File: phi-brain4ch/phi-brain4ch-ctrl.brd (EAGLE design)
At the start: 114.3 x 38.1 mm, 24 parts, among them U1 LCD-HD447804-HOLES16X2-4-HOLES

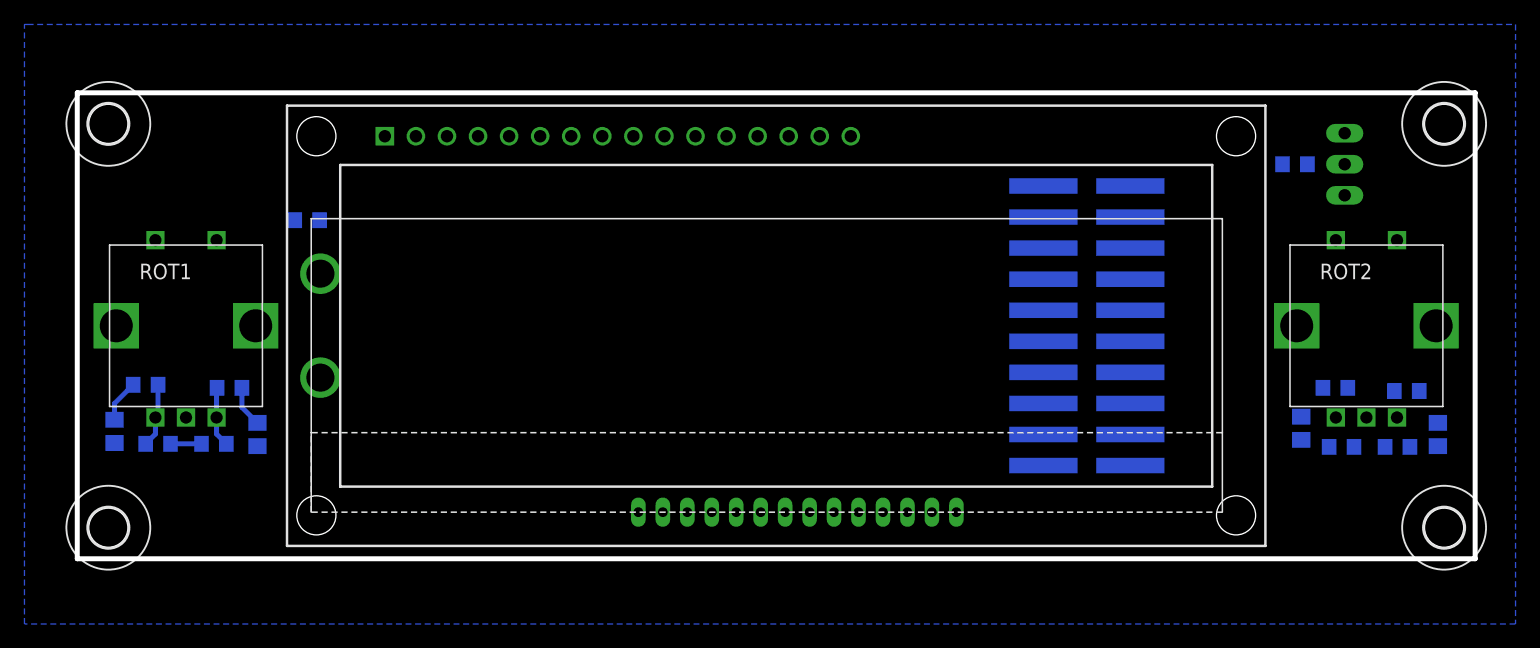
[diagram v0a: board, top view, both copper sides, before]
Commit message: wip
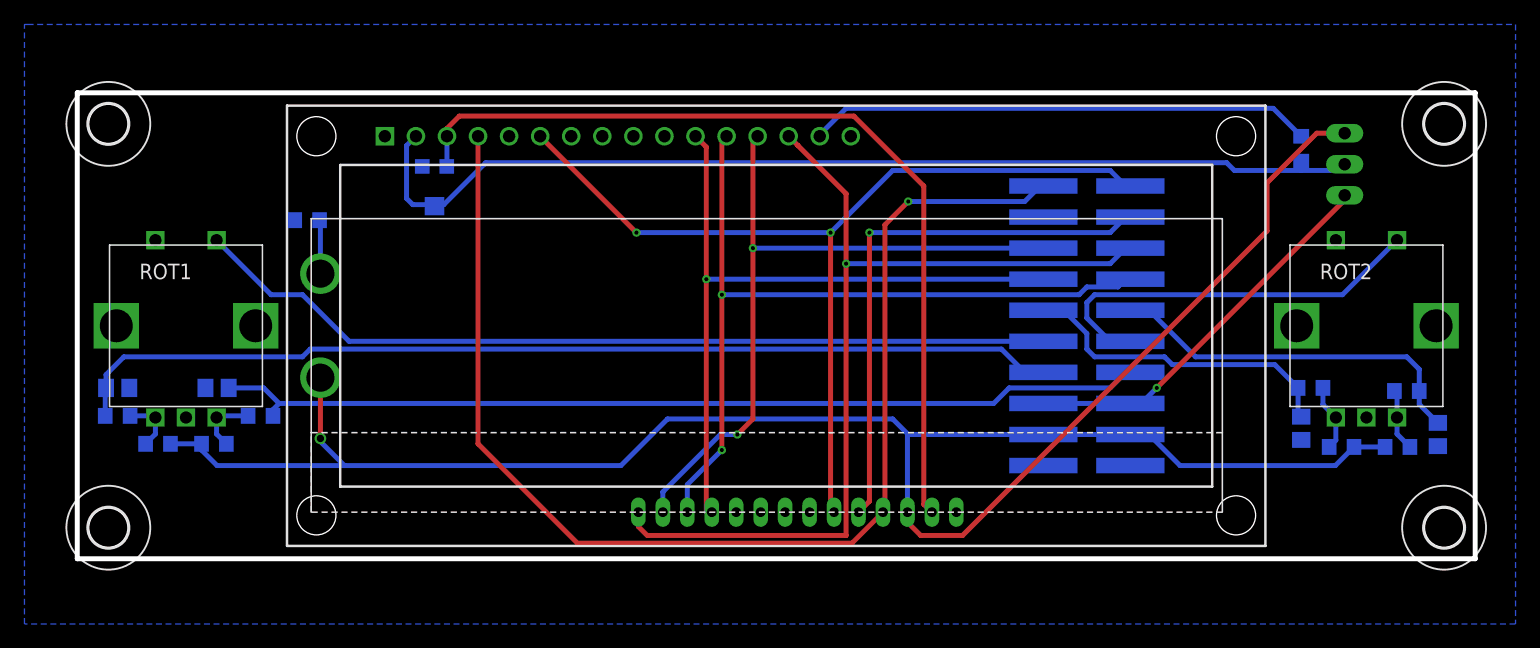
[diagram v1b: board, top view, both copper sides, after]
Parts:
- added VR1: 3303W-3-103E, microbuilder:TRIMPOT_BOURNS3MM
- moved C1 5.04 mm to (11.4, 14.0), turned to 0 degrees
- moved C2 3.57 mm to (3.30, 14.0), turned to 180 degrees
- moved R1 3.42 mm to (15.0, 11.7)
- moved R5 3.42 mm to (3.30, 11.7)
- moved R9 2.03 mm to (100.8, 14.0)
- moved R10 1.37 mm to (100.1, 33.5), turned to 270 degrees
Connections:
- net GND: now also VR1.A
- net LCD_V0: now also VR1.S
- net LCD_VDD: now also VR1.E
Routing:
- net 3.3V: track 2.54 -> 171.5 mm, vias 0 -> 1
- net LCD_RS: track 0.00 -> 100.5 mm, vias 0 -> 1
- net LCD_VDD: track 0.00 -> 85.2 mm
- net ROT1_A: track 3.49 -> 81.7 mm
- net LCD_EN: track 0.00 -> 77.1 mm, vias 0 -> 2
- net LCD_D7: track 0.00 -> 76.8 mm, vias 0 -> 1
- net ROT1_B: track 3.39 -> 76.5 mm
- net LCD_V0: track 0.00 -> 71.8 mm
- net ROT1_SW: track 0.00 -> 71.0 mm
- net LCD_D5: track 0.00 -> 66.0 mm, vias 0 -> 2
- net LCD_D4: track 0.00 -> 59.1 mm, vias 0 -> 1
- net LCD_D6: track 0.00 -> 58.5 mm, vias 0 -> 2
- net LCD_RW: track 0.00 -> 45.1 mm, vias 0 -> 1
- net N$6: track 0.00 -> 41.3 mm
- net ROT2_SW: track 0.00 -> 33.1 mm
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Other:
- board text added: "Designed by Eran Rundstein"
- board text added: "phi-brain-4ch-ctrl revision 1"
